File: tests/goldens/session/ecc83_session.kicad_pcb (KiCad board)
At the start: 2 copper layers, 40 x 30 mm, 15 parts

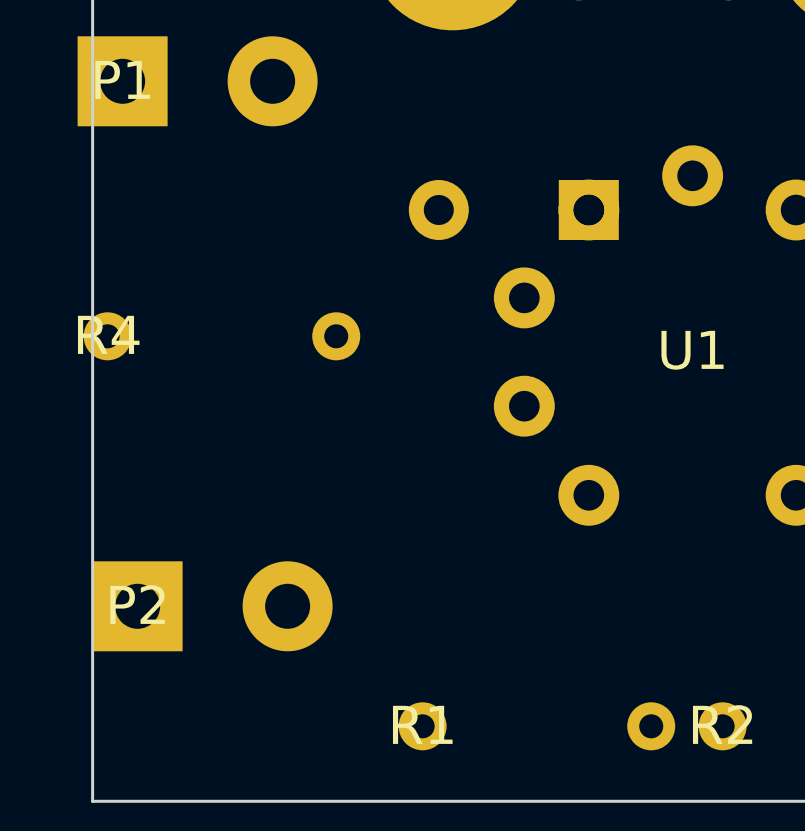
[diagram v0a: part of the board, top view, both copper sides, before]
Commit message: carve(v0.3.0): tree export at m3-signoff
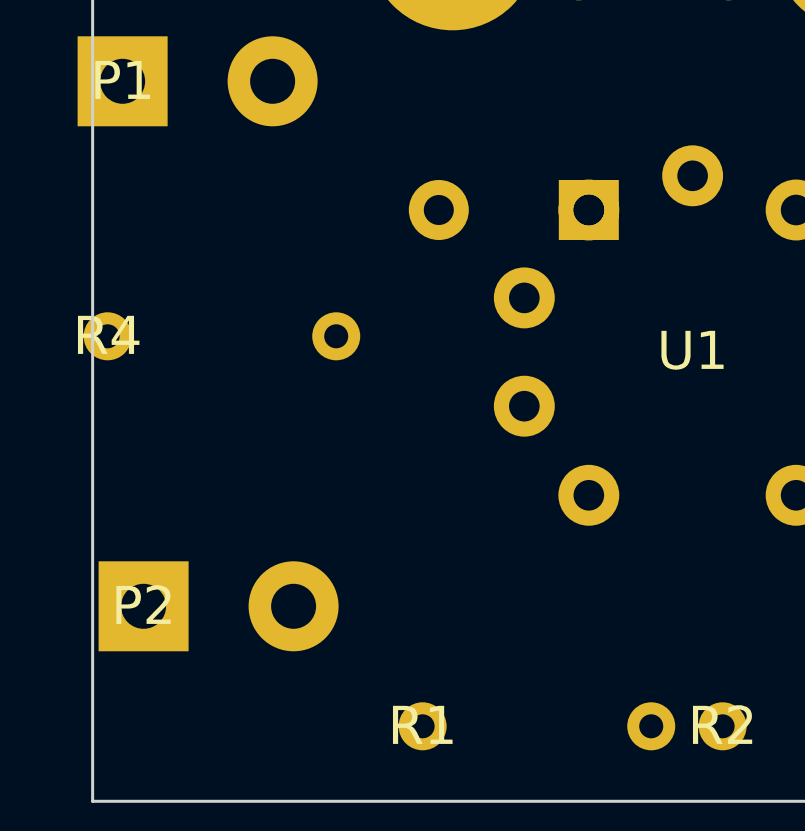
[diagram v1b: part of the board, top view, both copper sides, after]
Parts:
- moved P2 0.20 mm to (1.70, 23.5)
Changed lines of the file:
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@@
 		)
 		(pad "1" thru_hole rect
-			(at 0.000000 0.000000)
+			(at 0.000000 0.000000 180)
 			(size 2.000000 2.000000)
 			(drill 1.000000)
@@
 		)
 		(pad "2" thru_hole circle
-			(at -5.000000 0.000000)
+			(at -5.000000 0.000000 180)
 			(size 2.000000 2.000000)
 			(drill 1.000000)
@@
 	(footprint "Net2Board:Altech_AK300_1x02_P5.00mm_45-Degree"
 		(layer "F.Cu")
-		(at 1.500000 23.500000 0)
+		(at 1.699000 23.500000 0)
 		(property "Reference" "P2"
 			(at 0 0 0)
@@
 		)
 		(pad "1" thru_hole circle
-			(at 0.000000 0.000000)
+			(at 0.000000 0.000000 90)
 			(size 1.600000 1.600000)
 			(drill 0.800000)
@@
 		)
 		(pad "2" thru_hole oval
-			(at 7.620000 0.000000)
-			(size 1.600000 1.600000)
-			(drill 0.800000)
+			(at 7.620000 0.000000 90)
+			(size 1.600000 1.600000)
+			(drill 0.800000)
